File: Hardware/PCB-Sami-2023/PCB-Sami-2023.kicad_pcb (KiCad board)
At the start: 2 copper layers, 75 x 40 mm, 16 parts, among them J10 Bateria (+), J9 STEP_DOWN, P1 SensorTatamiDerecho, P2 SensorTatamiIzquierdo, P3 IFR_DER, P4 IFR_IZQ, P5 LDR, P6 MotorDerecho, P7 MotorIzquierdo, SW1 START, SW2 ESTRATEGIA, U1 ESP32-DEVKIT-V1

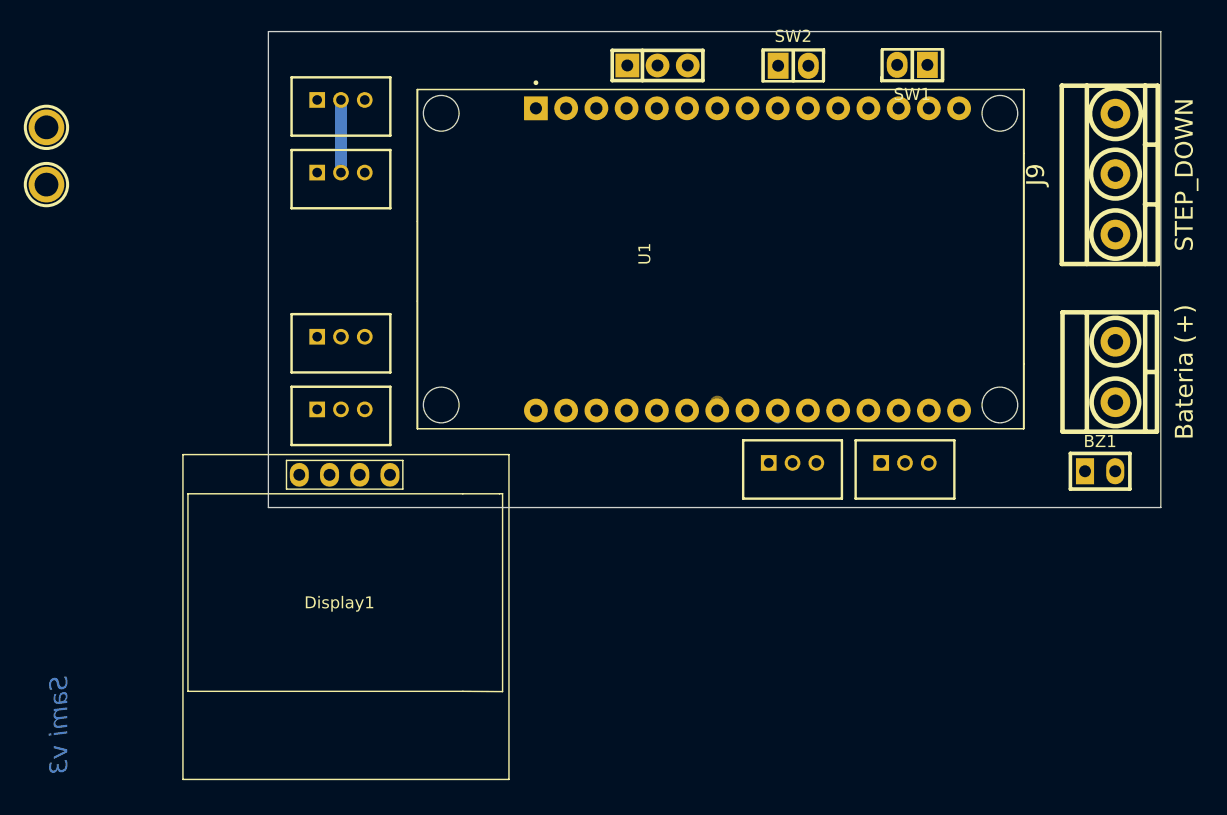
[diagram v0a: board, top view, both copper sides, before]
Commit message: placa terminada
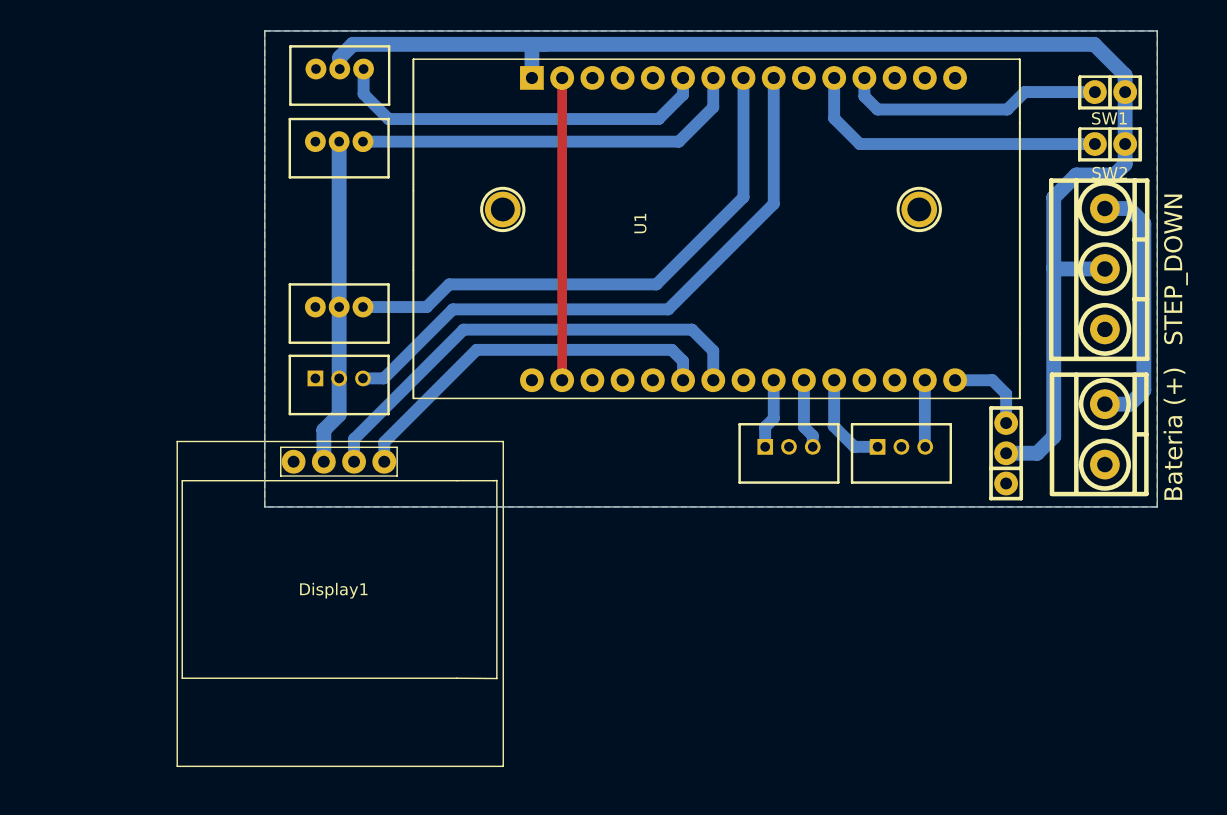
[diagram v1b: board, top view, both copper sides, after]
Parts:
- removed BZ1: Buzzer, EESTN5:Pin_strip_2
- moved H1 73.7 mm to (161.9, 66.8)
- moved P5 43.8 mm to (169.2, 87.3), turned to 90 degrees
- moved H2 38.4 mm to (126.9, 66.8)
- moved SW2 27.6 mm to (177.9, 61.6), turned to 180 degrees
- moved SW1 16.8 mm to (177.9, 57.3)
- moved J9 8.02 mm to (177.5, 71.8)
- moved J10 5.31 mm to (177.5, 85.7)
- moved P4 2.60 mm to (113.2, 61.1)
- moved P2 2.60 mm to (113.2, 81.0)
- moved P3 2.60 mm to (113.2, 55.0)
- moved U1 2.57 mm to (144.9, 68.0)
- moved P1 2.50 mm to (113.2, 75.0)
- moved P7 1.38 mm to (150.9, 86.8)
- moved P6 1.38 mm to (160.4, 86.8)
- moved Display1 1.20 mm to (112.9, 98.6)
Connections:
- U1 pad 10: /TATAMI_IZQ -> /BUZZER
- U1 pad 16: /BUZZER -> /LDR
- U1 pad 6: /IR_IZQ -> /IR_DER
- U1 pad 7: /IR_DER -> /IR_IZQ
- U1 pad 8: /LDR -> /TATAMI_DER
- U1 pad 9: /TATAMI_DER -> /TATAMI_IZQ
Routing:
- net +5V: track 6.10 -> 142.5 mm
- net /TATAMI_IZQ: track 0.00 -> 51.4 mm
- net /TATAMI_DER: track 0.00 -> 45.8 mm
- net /SCL: track 0.62 -> 39.1 mm
- net /IR_IZQ: track 0.00 -> 33.1 mm
- net /IR_DER: track 0.00 -> 32.1 mm
- net /SDA: track 0.22 -> 32.0 mm
- net /ESTRATEGIA: track 0.00 -> 26.2 mm
- net GND: track 0.00 -> 25.4 mm
- net /START: track 0.00 -> 22.4 mm
- net /Vstep: track 0.00 -> 21.6 mm
- net /M1A_PWM: track 0.00 -> 8.30 mm
- net /LDR: track 0.00 -> 7.22 mm
- net /M2B_DIR: track 0.00 -> 5.91 mm
- net /M1B_DIR: track 0.00 -> 5.61 mm
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- added copper zone on B.Cu, net GND
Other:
- board text removed: "Sami v3"
